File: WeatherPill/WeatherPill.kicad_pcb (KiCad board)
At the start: 2 copper layers, 95 x 32 mm, 27 parts, among them J2 Conn_02x08_Odd_Even, J3 USB4125-GF-A_REVA2, J4 Conn_02x08_Odd_Even, SW1 EVQ-P7A01P, SW2 EVQ-P7A01P, U1 STM32L052K8Tx, U12 USBLC6-2SC6, U13 BU9796AMUV-E2, U14 SHTC3, U2 SHT40-AD1B-R2, U3 BME280, U4 sst25vf512a-33-4c-sae, U7 STTS22HTR

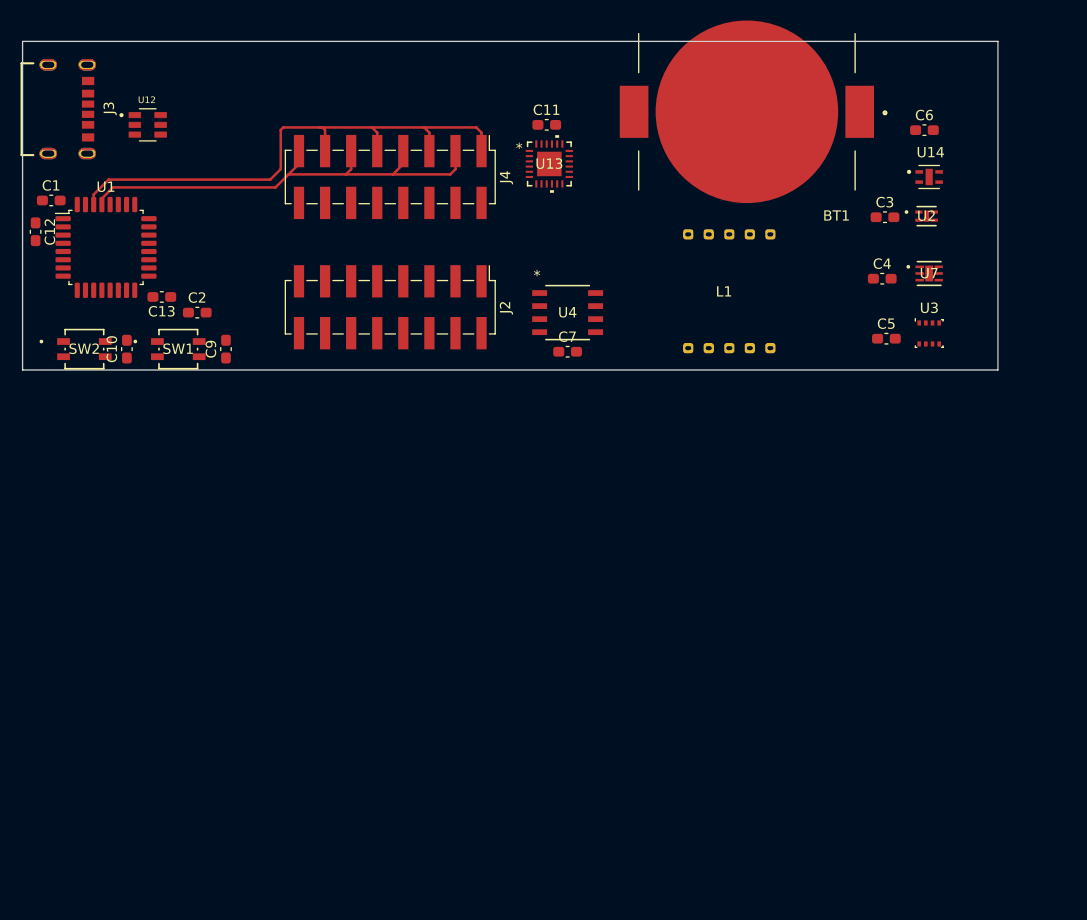
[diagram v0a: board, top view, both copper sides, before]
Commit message: in review
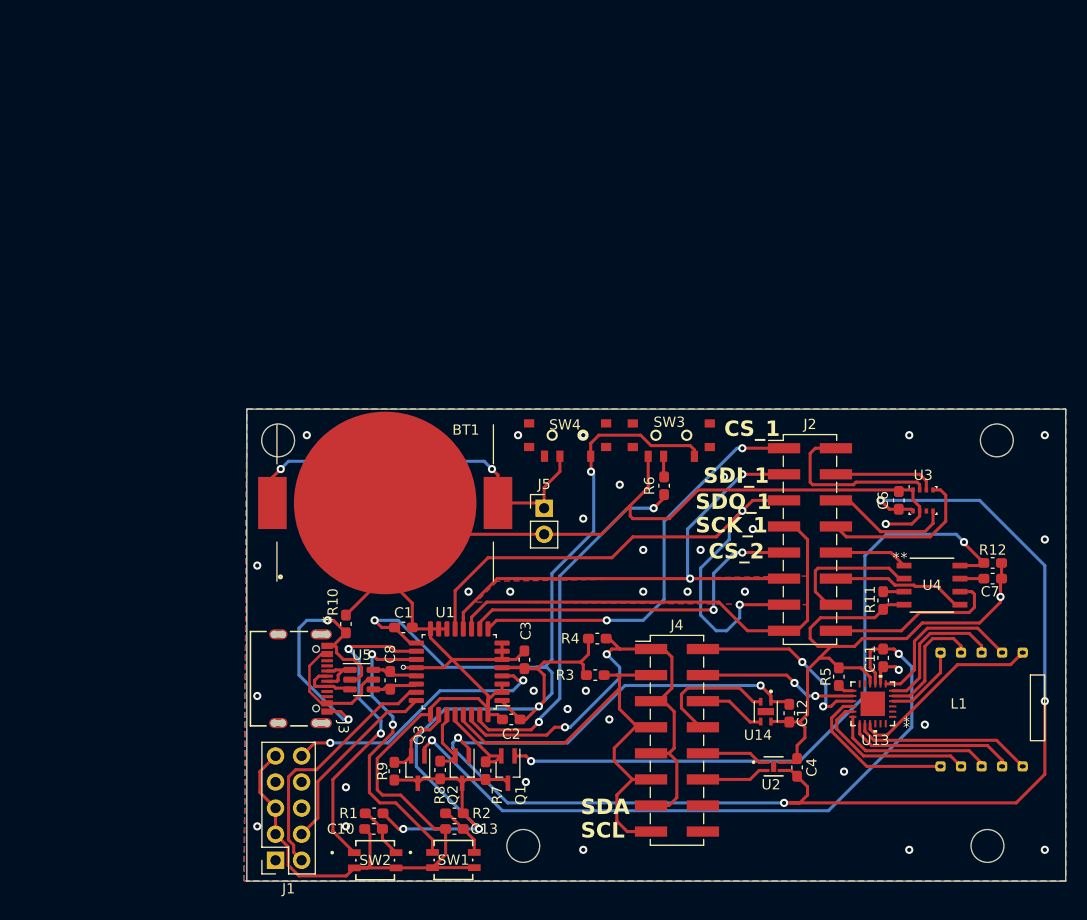
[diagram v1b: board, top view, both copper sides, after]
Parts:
- removed C5, C9: 0.1uF, Capacitor_SMD:C_0603_1608Metric_Pad1.08x0.95mm_HandSolder
- removed U12: USBLC6-2SC6, usb tvs:SOT95P280X145-6N
- removed U7: STTS22HTR, STTS22HTR:UDFN-6L_2X2X0P5_STM
- added C8: 100nF, Capacitor_SMD:C_0603_1608Metric_Pad1.08x0.95mm_HandSolder, F.Cu at (63.8, 157.2)
- added H1: MountingHole, MountingHole:MountingHole_3.2mm_M3_DIN965, F.Cu at (76.7, 173.4)
- added H2: MountingHole, MountingHole:MountingHole_3.2mm_M3_DIN965, F.Cu at (121.9, 173.4)
- added H3: MountingHole, MountingHole:MountingHole_3.2mm_M3_DIN965, F.Cu at (122.8, 133.9)
- added H4: MountingHole, MountingHole:MountingHole_3.2mm_M3_DIN965, F.Cu at (52.8, 133.9)
- added J1: Conn_02x05_Odd_Even, Connector_PinSocket_2.54mm:PinSocket_2x05_P2.54mm_Vertical, F.Cu at (52.6, 174.8)
- added J5: Conn_01x02_Pin, Connector_PinHeader_2.54mm:PinHeader_1x02_P2.54mm_Vertical, F.Cu at (78.7, 140.5)
- added Q1: PMOS, Package_TO_SOT_SMD:SOT-323_SC-70_Handsoldering, F.Cu at (75.2, 165.9)
- added Q2: PMOS, Package_TO_SOT_SMD:SOT-323_SC-70_Handsoldering, F.Cu at (70.8, 165.9)
- added Q3: PMOS, Package_TO_SOT_SMD:SOT-323_SC-70_Handsoldering, F.Cu at (66.4, 165.9)
- added R1: 1M, Capacitor_SMD:C_0603_1608Metric_Pad1.08x0.95mm_HandSolder, F.Cu at (62.2, 170.2)
- added R10: 0R, Capacitor_SMD:C_0603_1608Metric_Pad1.08x0.95mm_HandSolder, F.Cu at (59.4, 151.7)
- added R11: 0R, Capacitor_SMD:C_0603_1608Metric_Pad1.08x0.95mm_HandSolder, F.Cu at (111.8, 149.5)
- added R12: 0R, Capacitor_SMD:C_0603_1608Metric_Pad1.08x0.95mm_HandSolder, F.Cu at (122.4, 147.3)
- added R2: 1M, Capacitor_SMD:C_0603_1608Metric_Pad1.08x0.95mm_HandSolder, F.Cu at (70.0, 170.2)
- added R3: 10K, Capacitor_SMD:C_0603_1608Metric_Pad1.08x0.95mm_HandSolder, F.Cu at (83.7, 156.7)
- added R4: 10K, Capacitor_SMD:C_0603_1608Metric_Pad1.08x0.95mm_HandSolder, F.Cu at (83.9, 153.2)
- added R5: 0R, Capacitor_SMD:C_0603_1608Metric_Pad1.08x0.95mm_HandSolder, F.Cu at (107.4, 156.9)
- added R6: 10K, Capacitor_SMD:C_0603_1608Metric_Pad1.08x0.95mm_HandSolder, F.Cu at (90.4, 138.3)
- added R7: 1M, Capacitor_SMD:C_0603_1608Metric_Pad1.08x0.95mm_HandSolder, F.Cu at (73.0, 166.0)
- added R8: 1M, Capacitor_SMD:C_0603_1608Metric_Pad1.08x0.95mm_HandSolder, F.Cu at (68.6, 166.0)
- added R9: 1M, Capacitor_SMD:C_0603_1608Metric_Pad1.08x0.95mm_HandSolder, F.Cu at (64.2, 166.1)
- added SW3: SW_DPDT_x2, dpdt_switch:450404015514, F.Cu at (91.1, 133.4)
- added SW4: SW_DPDT_x2, dpdt_switch:450404015514, F.Cu at (81.0, 133.3)
- added U5: USBLC6-2SC6, Package_TO_SOT_SMD:SOT-23-6, F.Cu at (61.0, 157.2)
- C10, C11, C13, C4, C6: value 0.1uF -> 100nF
- J3: value USB4125-GF-A_REVA2 -> 12402012E212A; footprint usb con:GCT_USB4125-GF-A_REVA2 -> usb conn:12402012E212A_AMP
- moved C12 87.1 mm to (102.6, 160.4), turned to 90 degrees
- moved J4 61.6 mm to (91.7, 163.1), turned to 0 degrees
- moved C11 61.4 mm to (111.8, 155.0), turned to 90 degrees
- moved U13 61.3 mm to (110.7, 159.5)
- moved J3 59.9 mm to (53.9, 157.1)
- moved C13 59.1 mm to (70.0, 171.7), turned to 0 degrees
- moved SW2 57.3 mm to (62.3, 174.8)
- moved SW1 56.5 mm to (69.9, 174.7)
- moved U2 55.6 mm to (101.1, 165.6)
- moved C3 55.6 mm to (76.8, 155.2), turned to 90 degrees
- moved U14 54.4 mm to (100.3, 160.3), turned to -90 degrees
- moved C1 53.9 mm to (65.0, 152.1)
- moved U1 53.8 mm to (70.5, 156.4), turned to 180 degrees
- moved C10 52.6 mm to (62.1, 171.7), turned to 0 degrees
- moved BT1 51.9 mm to (63.3, 140.0), turned to 0 degrees
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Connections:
- net Net-(J2-Pin_10) renamed CS_SST25
- net Net-(J2-Pin_12) renamed SDI_SST25
- net Net-(J2-Pin_14) renamed SDO_SST25
- net Net-(J2-Pin_16) renamed SCK_SST25
- net Net-(J2-Pin_2) renamed CS_BME280
- net Net-(J2-Pin_4) renamed SDI_BME280
- net Net-(J4-Pin_10) renamed SDA_SHT40
- net Net-(J4-Pin_12) renamed SCL_SHT40
- net Net-(J4-Pin_2) renamed SDA_DISPLAY
- net Net-(J4-Pin_4) renamed SCL_DISPLAY
- net Net-(J4-Pin_6) renamed SDA_SHTC3
- net Net-(J4-Pin_8) renamed SCL_SHTC3
- BT1 pad 1: V_BUS_3V -> Net-(J5-Pin_1)
- BT1 pad 2: V_BUS_3V -> Net-(J5-Pin_1)
- C10 pad 2: V_BUS_3V -> Net-(C10-Pad2)
- C11 pad 2: V_BUS_3V -> V_BUS_ZONE_3
- C12 pad 2: V_BUS_3V -> V_BUS_ZONE_2
- C13 pad 2: V_BUS_3V -> Net-(C13-Pad2)
- C4 pad 2: V_BUS_3V -> V_BUS_ZONE_2
- C6 pad 2: V_BUS_3V -> V_BUS_ZONE_2
- C7 pad 2: V_BUS_3V -> V_BUS_ZONE_1
- J2 pad 6: Net-(J2-Pin_6) -> SDO_BME280
- J2 pad 8: Net-(J2-Pin_8) -> SCK_BME280
- J4 pad 14: Net-(J4-Pin_14) -> unconnected-(J4-Pin_14-Pad14)
- J4 pad 16: Net-(J4-Pin_16) -> unconnected-(J4-Pin_16-Pad16)
- L1 pad 1: unconnected-(L1-Pad1) -> Net-(L1-0)
- L1 pad 10: unconnected-(L1-Pad10) -> Net-(L1-A)
- L1 pad 2: unconnected-(L1-Pad2) -> Net-(L1-1)
- L1 pad 3: unconnected-(L1-Pad3) -> Net-(L1-2)
- L1 pad 4: unconnected-(L1-Pad4) -> Net-(L1-3)
- L1 pad 5: unconnected-(L1-Pad5) -> Net-(L1-4)
- L1 pad 6: unconnected-(L1-Pad6) -> Net-(L1-E)
- L1 pad 7: unconnected-(L1-Pad7) -> Net-(L1-D)
- L1 pad 8: unconnected-(L1-Pad8) -> Net-(L1-C)
- L1 pad 9: unconnected-(L1-Pad9) -> Net-(L1-B)
- SW1 pad 1: BTN_0 -> BTN_1
- SW1 pad 1*: V_BUS_3V -> Net-(C13-Pad2)
- SW2 pad 1: BTN_1 -> BTN_2
- SW2 pad 1*: V_BUS_3V -> Net-(C10-Pad2)
- U1 pad 14: BTN_0 -> GND
- U1 pad 15: BTN_1 -> GND
- U1 pad 18: unconnected-(U1-PA8-Pad18) -> BTN_2
- U1 pad 19: unconnected-(U1-PA9-Pad19) -> BTN_1
- U1 pad 2: unconnected-(U1-PC14-Pad2) -> GND
- U1 pad 20: unconnected-(U1-PA10-Pad20) -> GND
- U1 pad 21: unconnected-(U1-PA11-Pad21) -> USB_D-
- U1 pad 22: unconnected-(U1-PA12-Pad22) -> USB_D+
- U1 pad 23: unconnected-(U1-PA13-Pad23) -> SWDIO
- U1 pad 24: unconnected-(U1-PA14-Pad24) -> SWCLK
- U1 pad 25: unconnected-(U1-PA15-Pad25) -> GND
- U1 pad 26: unconnected-(U1-PB3-Pad26) -> CONTROL_ZONE_3
- U1 pad 27: unconnected-(U1-PB4-Pad27) -> CONTROL_ZONE_2
- U1 pad 28: unconnected-(U1-PB5-Pad28) -> CONTROL_ZONE_1
- U1 pad 3: unconnected-(U1-PC15-Pad3) -> GND
- U1 pad 31: unconnected-(U1-BOOT0-Pad31) -> BOOT
- U1 pad 6: unconnected-(U1-PA0-Pad6) -> GND
- U1 pad 7: unconnected-(U1-PA1-Pad7) -> GND
- U1 pad 8: unconnected-(U1-PA2-Pad8) -> GND
- U13 pad 1: unconnected-(U13-OSCIN-Pad1) -> Net-(U13-OSCIN)
- U13 pad 16: unconnected-(U13-COM0-Pad16) -> Net-(L1-A)
- U13 pad 17: unconnected-(U13-COM1-Pad17) -> Net-(L1-B)
- U13 pad 18: unconnected-(U13-COM2-Pad18) -> Net-(L1-C)
- U13 pad 19: unconnected-(U13-COM3-Pad19) -> Net-(L1-D)
- U13 pad 20: unconnected-(U13-VLCD-Pad20) -> GND
- U13 pad 21: V_BUS_3V -> V_BUS_ZONE_3
- U13 pad 4: unconnected-(U13-SEG0-Pad4) -> Net-(L1-0)
- U13 pad 5: unconnected-(U13-SEG1-Pad5) -> Net-(L1-1)
- U13 pad 6: unconnected-(U13-SEG2-Pad6) -> Net-(L1-2)
- U13 pad 7: unconnected-(U13-SEG3-Pad7) -> Net-(L1-3)
- U13 pad 8: unconnected-(U13-SEG4-Pad8) -> Net-(L1-4)
- U13 pad 9: unconnected-(U13-SEG5-Pad9) -> Net-(L1-E)
- U14 pad 1: V_BUS_3V -> V_BUS_ZONE_2
- U2 pad 3: V_BUS_3V -> V_BUS_ZONE_2
- U3 pad 4: Net-(J2-Pin_6) -> SCK_BME280
- U3 pad 5: Net-(J2-Pin_8) -> SDO_BME280
- U3 pad 8: V_BUS_3V -> V_BUS_ZONE_2
- U4 pad 3: unconnected-(U4-*WP-Pad3) -> Net-(U4-*WP)
- U4 pad 7: unconnected-(U4-*HOLD-Pad7) -> Net-(U4-*HOLD)
- U4 pad 8: V_BUS_3V -> V_BUS_ZONE_1
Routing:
- net GND: track 0.00 -> 265.9 mm, vias 0 -> 36
- net V_BUS_ZONE_2: track 0.00 -> 149.5 mm, vias 0 -> 5
- net V_BUS_3V: track 0.00 -> 138.5 mm, vias 0 -> 5
- net V_BUS_ZONE_3: track 0.00 -> 68.9 mm, vias 0 -> 2
- net V_BUS_ZONE_1: track 0.00 -> 66.7 mm, vias 0 -> 2
- net SDO_1: track 0.00 -> 61.8 mm, vias 0 -> 2
- net SDI_1: track 0.00 -> 50.7 mm, vias 0 -> 2
- net SCK_1: track 0.00 -> 46.7 mm
- net CS_1: track 0.00 -> 40.6 mm, vias 0 -> 2
- net Net-(J5-Pin_1): track 0.00 -> 38.8 mm, vias 0 -> 2
- net BOOT: track 0.00 -> 35.7 mm, vias 0 -> 2
- net CS_2: track 0.00 -> 35.2 mm, vias 0 -> 2
- net BTN_2: track 0.00 -> 31.0 mm, vias 0 -> 2
- net BTN_1: track 0.00 -> 29.1 mm, vias 0 -> 2
- net Net-(U5-GND): track 0.00 -> 27.9 mm, vias 0 -> 2
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- added copper zone on B.Cu, net GND
- added copper zone on F.Cu, net GND
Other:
- board size 95 x 32 mm -> 79.8 x 46 mm
- board text added: "CS_1"
- board text added: "CS_2"
- board text added: "SCK_1"
- board text added: "SCL"
- board text added: "SDA"
- board text added: "SDI_1"
- board text added: "SDO_1"
